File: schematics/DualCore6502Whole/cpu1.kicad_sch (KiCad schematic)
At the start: 5 parts, among them U2 W65C02S

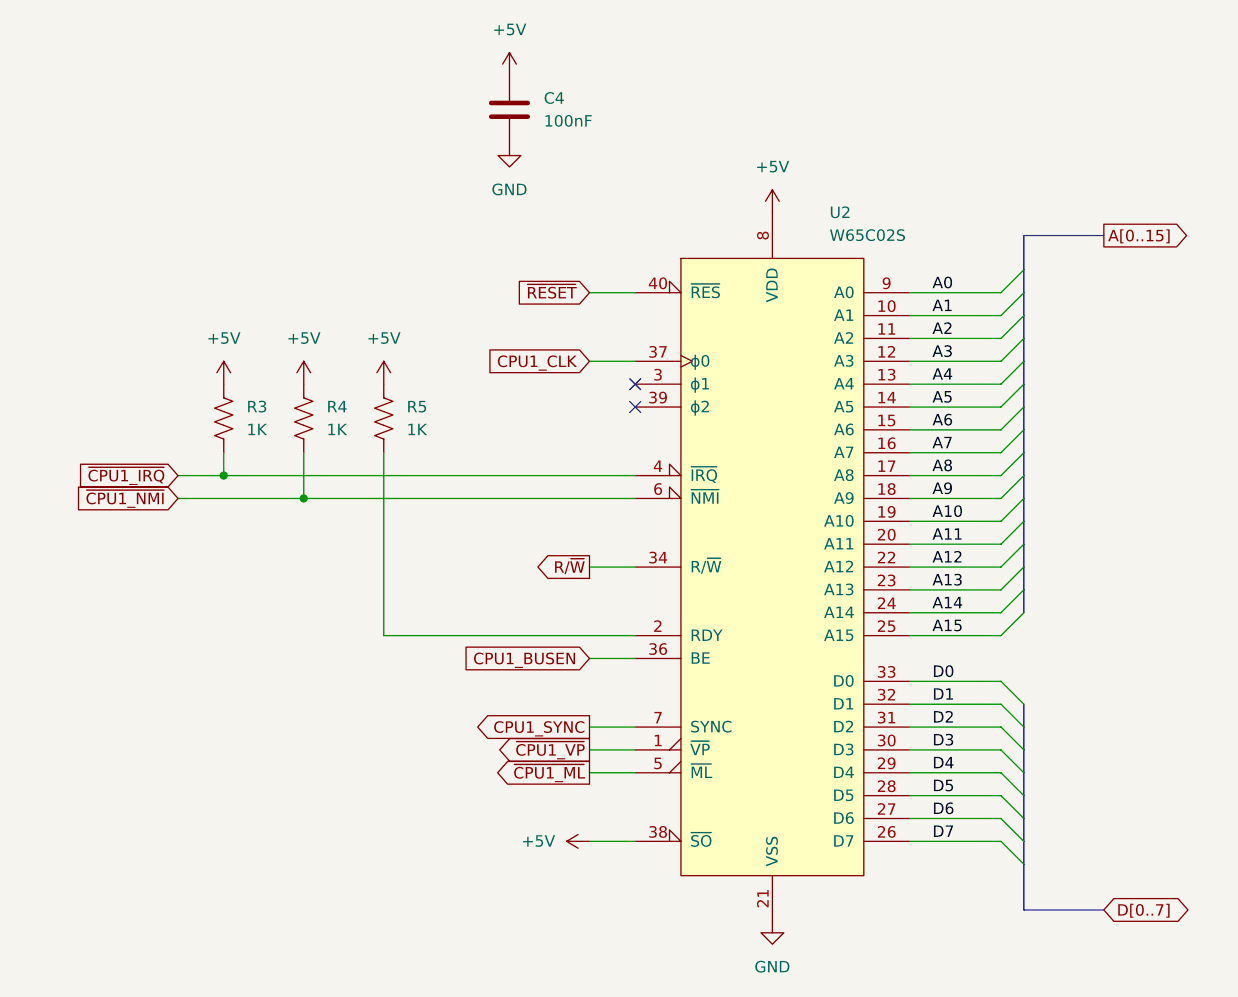
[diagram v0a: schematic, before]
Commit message: Basic PCB layout
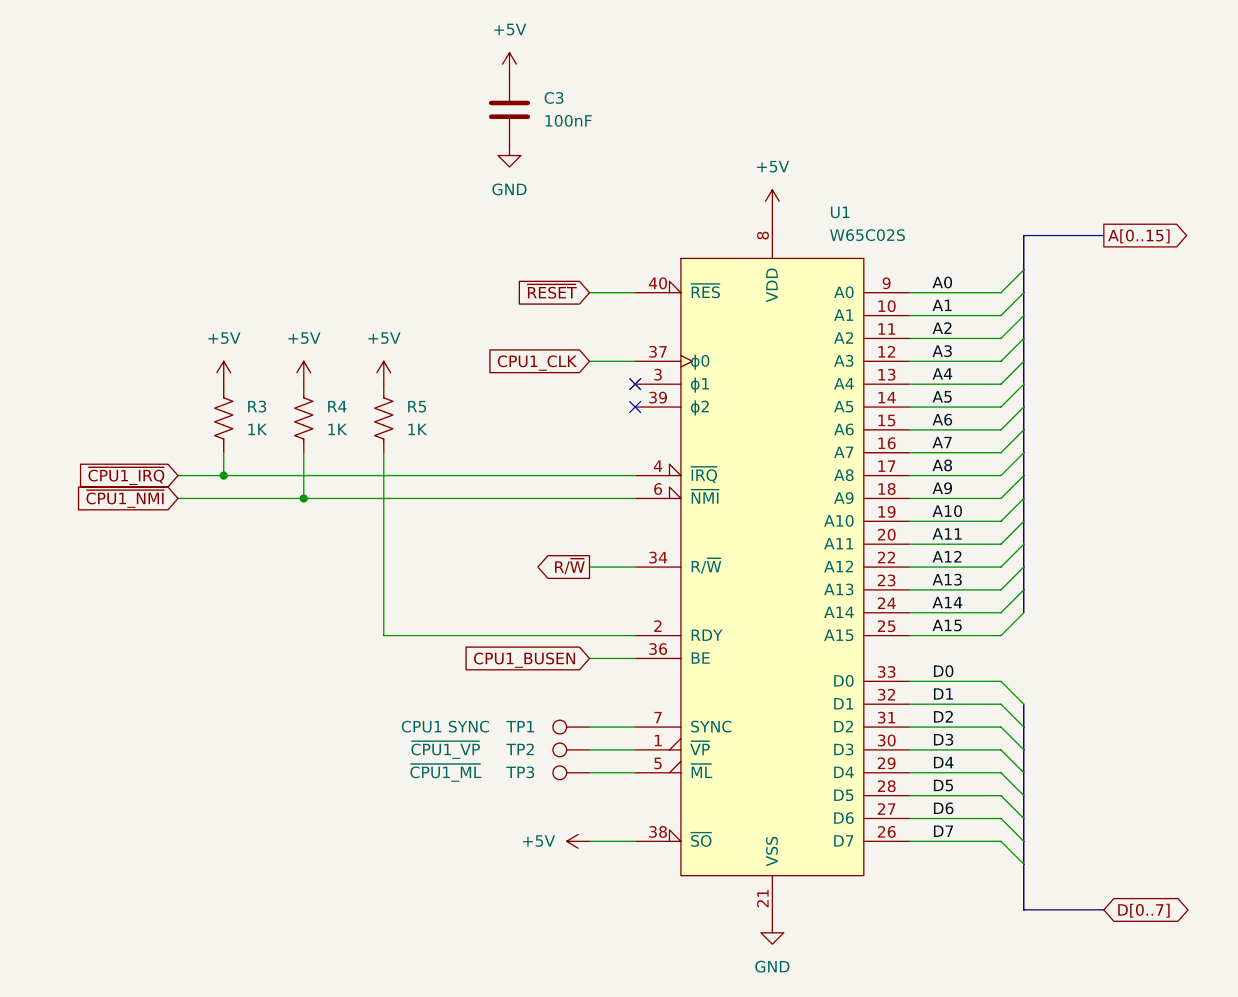
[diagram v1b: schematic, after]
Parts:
- added TP1: CPU1 SYNC, TestPoint:TestPoint_Pad_D1.5mm, symbol Connector:TestPoint
- added TP2: ~{CPU1_VP}, TestPoint:TestPoint_Pad_D1.5mm, symbol Connector:TestPoint
- added TP3: ~{CPU1_ML}, TestPoint:TestPoint_Pad_D1.5mm, symbol Connector:TestPoint
- U1: renamed from U2; footprint Package_DIP:DIP-40_W15.24mm -> Package_DIP:DIP-40_W15.24mm_Socket
- renumbered C4 to C3
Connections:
- net CPU1_SYNC: no longer names the net of U1.7 (SYNC)
- net CPU1_SYNC: now also TP1.1
- net ~{CPU1_ML}: no longer names the net of U1.5 (~{ML})
- net ~{CPU1_ML}: now also TP3.1
- net ~{CPU1_VP}: no longer names the net of U1.1 (~{VP})
- net ~{CPU1_VP}: now also TP2.1
